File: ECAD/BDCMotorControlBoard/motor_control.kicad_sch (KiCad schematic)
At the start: 30 parts, among them J1 Motor Connector, J4 Limit switch, J5 Limit switch, U10 PGA112, U2 DRV8870DDA, U3 INA180A1

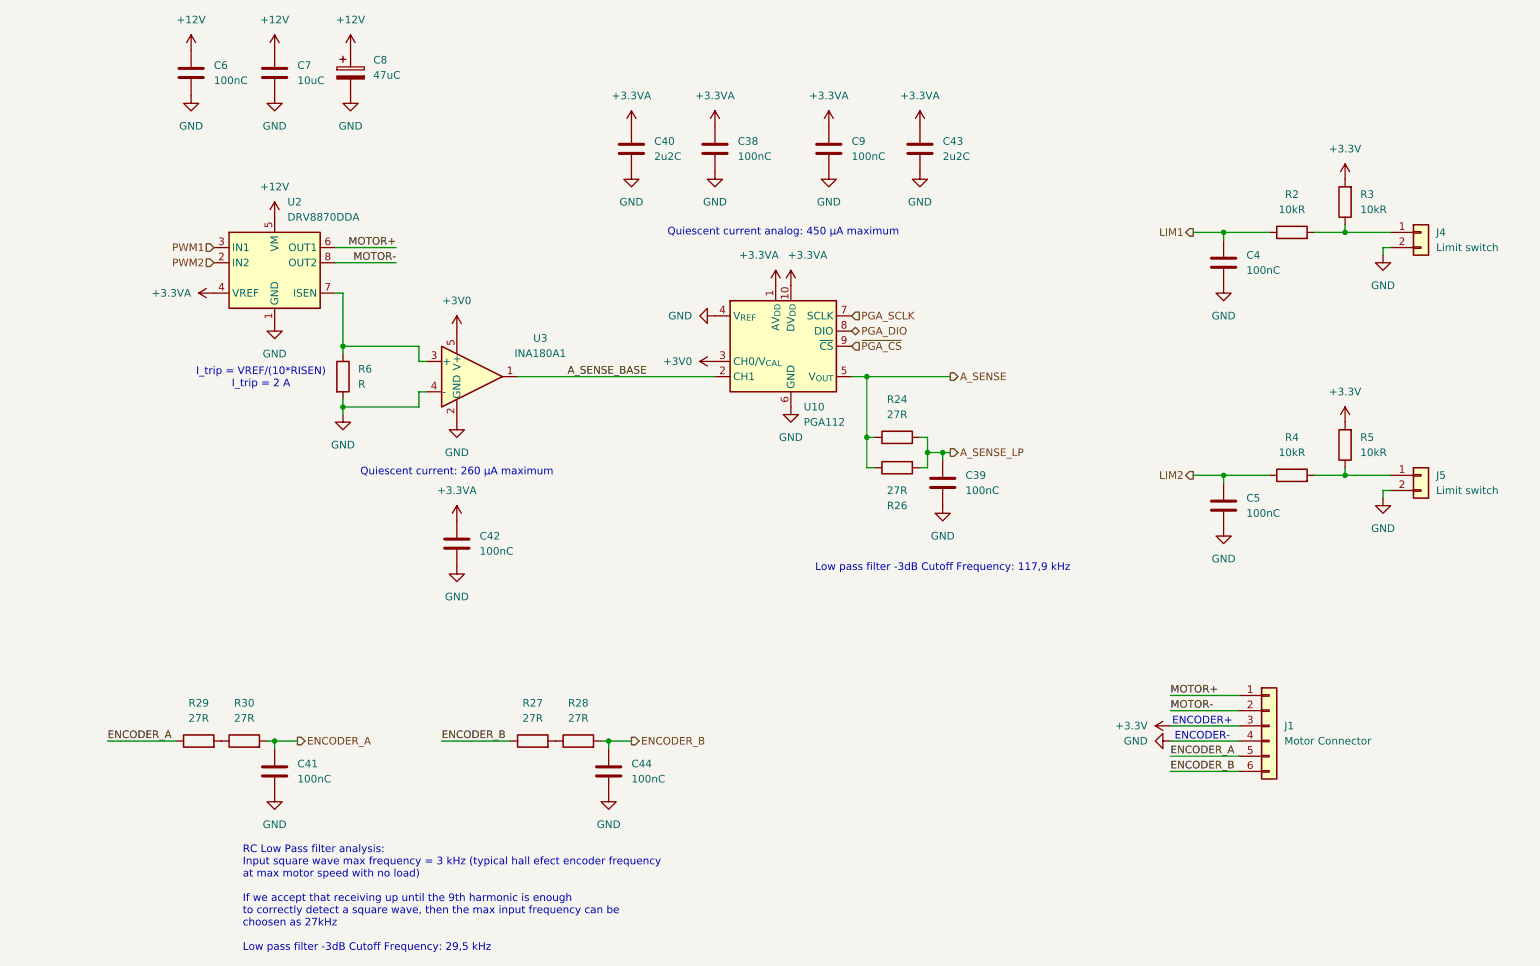
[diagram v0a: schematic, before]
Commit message: Progressed ECAD.
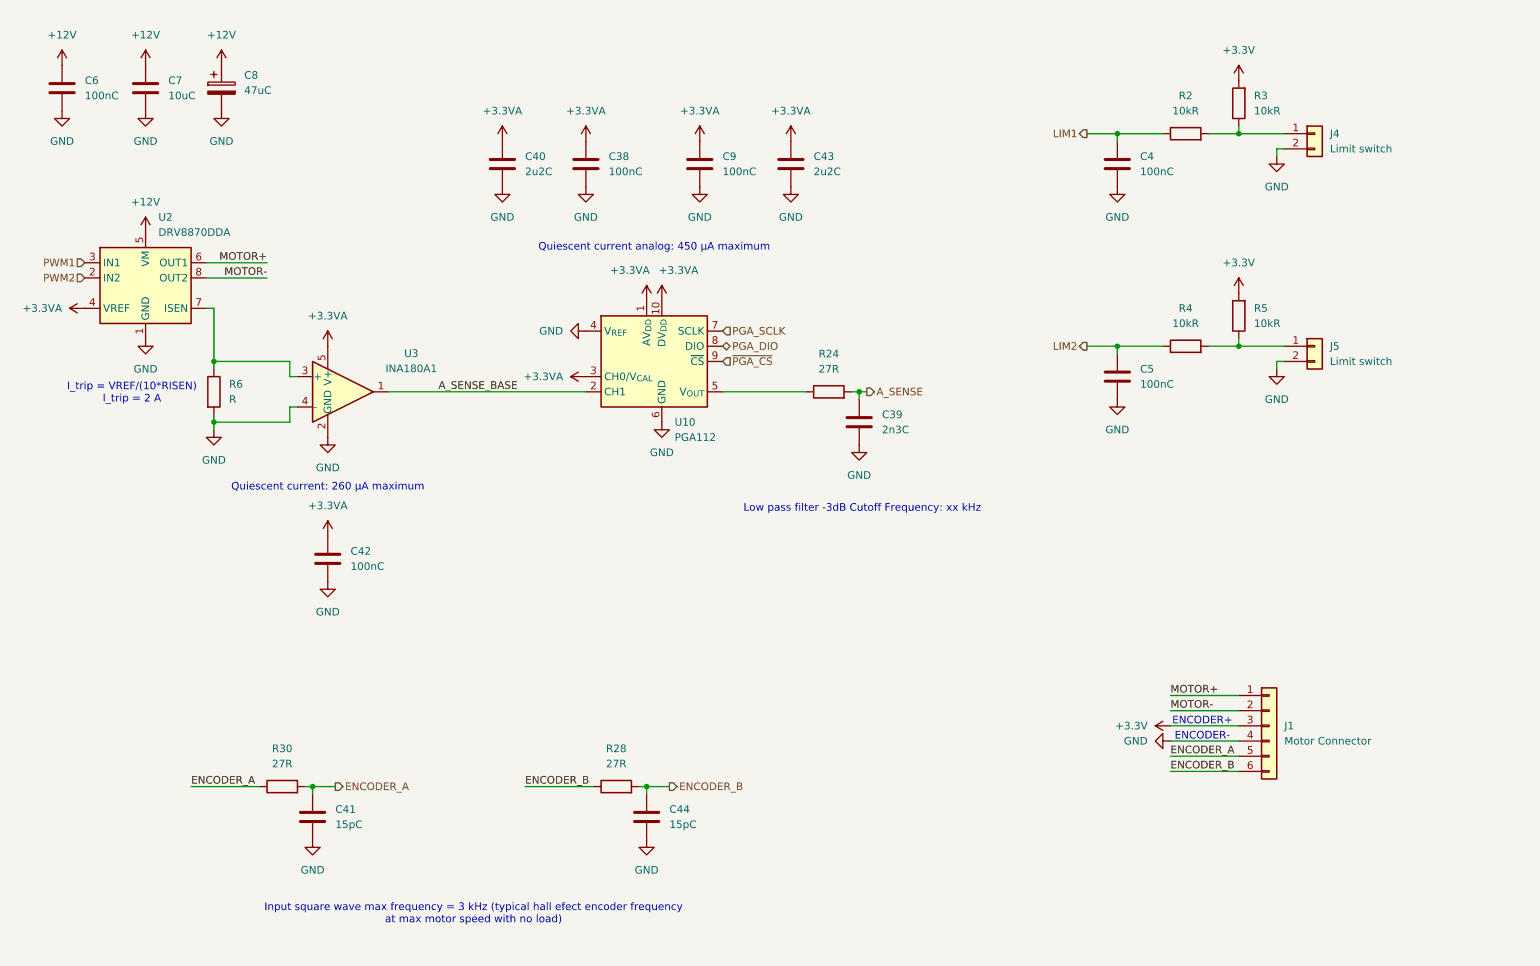
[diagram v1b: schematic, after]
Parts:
- removed R26, R27, R29: 27R, Resistor_SMD:R_0201_0603Metric, symbol Device:R
- C39: value 100nC -> 2n3C
- C41, C44: value 100nC -> 15pC; footprint (none) -> Capacitor_SMD:C_0201_0603Metric; MPN (none) -> GRM0335C1E150JA01D
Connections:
- net +3V0 is gone; now on net +3.3VA: U10.3 (CH0/V_{CAL}), U3.5 (V+)
- net A_SENSE_LP is gone; now on net A_SENSE: C39.1, R24.2
- net A_SENSE: no longer R24.1, U10.5 (V_{OUT})
- net ENCODER_A: now also C41.2, R30.1; no longer C41.1
- net ENCODER_B: now also C44.2, R28.1; no longer C44.1
- net GND: now also C41.1, C44.1; no longer C41.2, C44.2
- new net: R24.1, U10.5 (V_{OUT})
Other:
- note added: "Input square wave max frequency = 3 kHz (typical hall efect encoder frequency at max motor speed with no load)"
- note added: "Low pass filter -3dB Cutoff Frequency: xx kHz"
- note removed: "Low pass filter -3dB Cutoff Frequency: 117,9 kHz"
- note removed: "RC Low Pass filter analysis: Input square wave max frequency = 3 kHz (typical hall efect encoder frequency at max motor speed with no load) If we accept that receiving up until the 9th harmonic is enough to correctly detect a square wave, then the max input frequency can be choosen as 27kHz Low pass filter -3dB Cutoff Frequency: 29,5 kHz"
- moved on the sheet: C38, C39, C4, C40, C42, C43, C5, C6, C7, C8, C9, J4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
